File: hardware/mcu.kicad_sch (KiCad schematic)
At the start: 30 parts, among them J9 Conn_ARM_JTAG_SWD_10, Q1 MMBT3904, Q2 MMBT3904, Q3 MMBT3904, SW1 SW_Push, SW2 SW_Push, U3 STM32L476RGTx, Y1 DNP

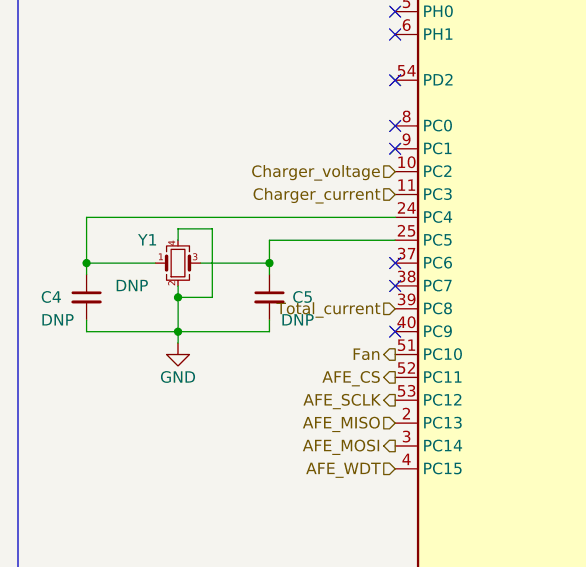
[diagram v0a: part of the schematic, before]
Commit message: Initiated sourcing
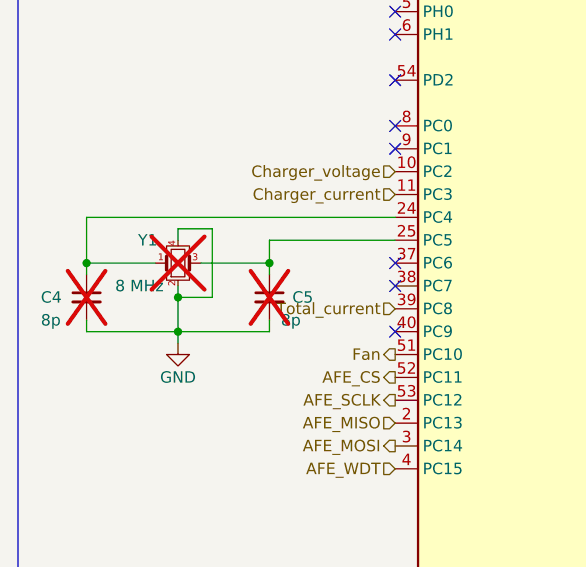
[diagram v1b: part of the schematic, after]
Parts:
- C4, C5: value DNP -> 8p; now not fitted
- Y1: value DNP -> 8 MHz; now not fitted
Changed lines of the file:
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@@
 		(in_bom yes)
 		(on_board yes)
-		(dnp no)
+		(dnp yes)
 		(property "Reference" "Y1"
 			(at 41.275 87.63 0)
@@
 			)
 		)
-		(property "Value" "DNP"
+		(property "Value" "8 MHz"
 			(at 38.735 92.71 0)
 			(effects
@@
 		(in_bom yes)
 		(on_board yes)
-		(dnp no)
+		(dnp yes)
 		(property "Reference" "C4"
 			(at 30.48 93.98 0)
@@
 			)
 		)
-		(property "Value" "DNP"
+		(property "Value" "8p"
 			(at 30.48 96.52 0)
 			(effects
@@
 		(in_bom yes)
 		(on_board yes)
-		(dnp no)
+		(dnp yes)
 		(property "Reference" "C5"
 			(at 58.42 93.98 0)
@@
 			)
 		)
-		(property "Value" "DNP"
+		(property "Value" "8p"
 			(at 57.15 96.52 0)
 			(effects

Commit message: More sourcing components
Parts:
- D1: footprint LED_THT:LED_D3.0mm -> LED_THT:LED_D5.0mm; LCSC (none) -> C2895548
- D2: footprint LED_THT:LED_D3.0mm -> LED_THT:LED_D5.0mm; LCSC (none) -> C2895492
- R2, R4, R7: footprint (none) -> Resistor_SMD:R_0402_1005Metric
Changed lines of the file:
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@@
 			)
 		)
-		(property "Footprint" ""
+		(property "Footprint" "Resistor_SMD:R_0402_1005Metric"
 			(at 247.65 144.78 0)
 			(effects
@@
 			)
 		)
-		(property "Footprint" "LED_THT:LED_D3.0mm"
+		(property "Footprint" "LED_THT:LED_D5.0mm"
 			(at 209.55 132.08 90)
 			(effects
@@
 		(property "Description" ""
 			(at 209.55 132.08 0)
+			(effects
+				(font
+					(size 1.27 1.27)
+				)
+				(hide yes)
+			)
+		)
+		(property "LCSC" "C2895492"
+			(at 209.55 132.08 90)
 			(effects
 				(font
@@
 			)
 		)
-		(property "Footprint" "LED_THT:LED_D3.0mm"
+		(property "Footprint" "LED_THT:LED_D5.0mm"
 			(at 171.45 132.08 90)
 			(effects
@@
 			)
 		)
+		(property "LCSC" "C2895548"
+			(at 171.45 132.08 90)
+			(effects
+				(font
+					(size 1.27 1.27)
+				)
+				(hide yes)
+			)
+		)
 		(pin "1"
 		)
@@
 			)
 		)
-		(property "Footprint" ""
+		(property "Footprint" "Resistor_SMD:R_0402_1005Metric"
 			(at 198.12 147.32 0)
 			(effects
@@
 			)
 		)
-		(property "Footprint" ""
+		(property "Footprint" "Resistor_SMD:R_0402_1005Metric"
 			(at 160.02 147.32 0)
 			(effects

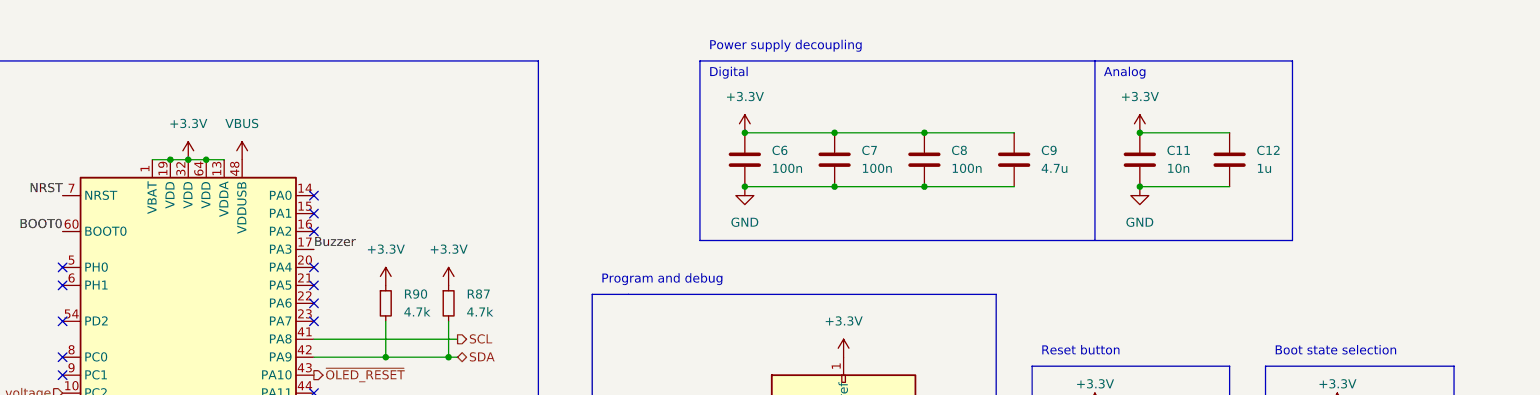
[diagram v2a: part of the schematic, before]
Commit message: Improved Currrent Sensors
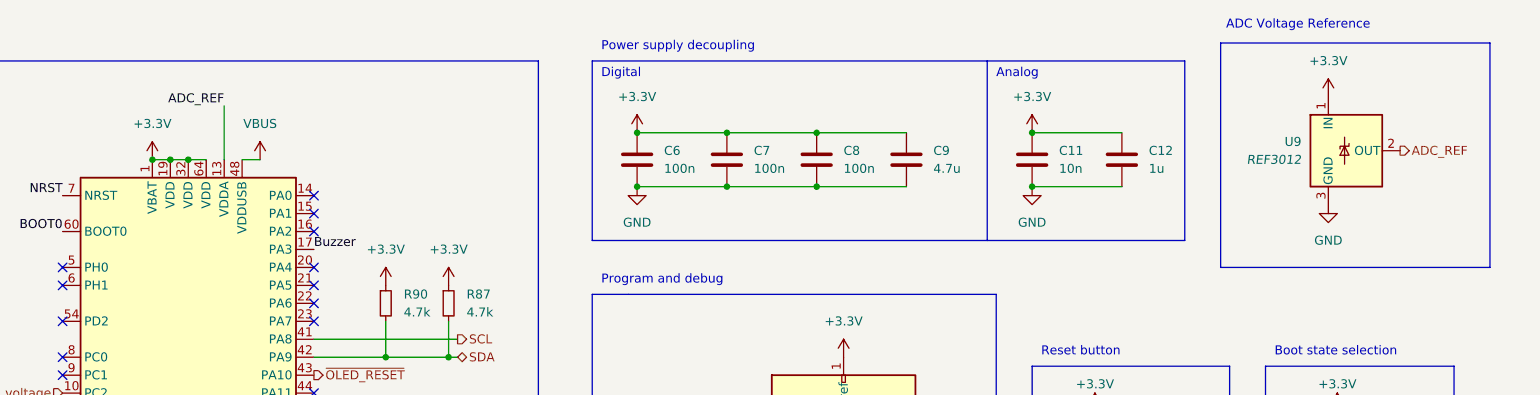
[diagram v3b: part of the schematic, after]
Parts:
- added U9: REF3012, Package_TO_SOT_SMD:SOT-23, symbol Reference_Voltage:REF3012
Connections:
- net +3.3V: now also U9.1 (IN); no longer U3.13 (VDDA)
- net GND: now also U9.3 (GND)
- new net ADC_REF: U3.13 (VDDA), U9.2 (OUT)
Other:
- note added: "ADC Voltage Reference"
- moved on the sheet: C11, C12, C6, C7, C8, C9

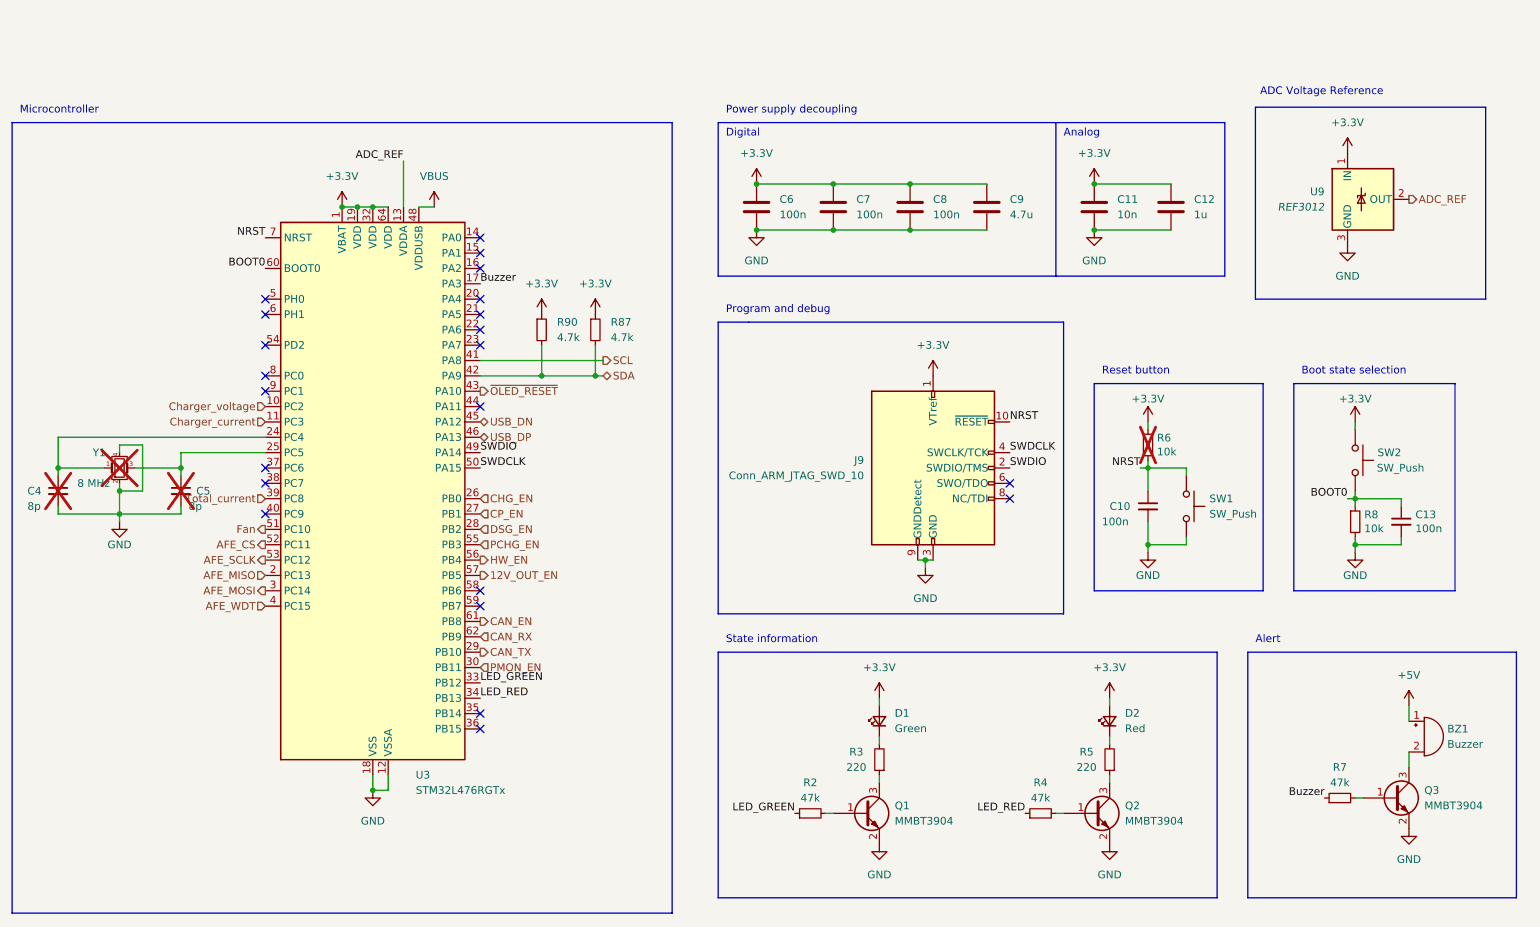
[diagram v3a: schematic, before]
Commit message: Charger monitoring
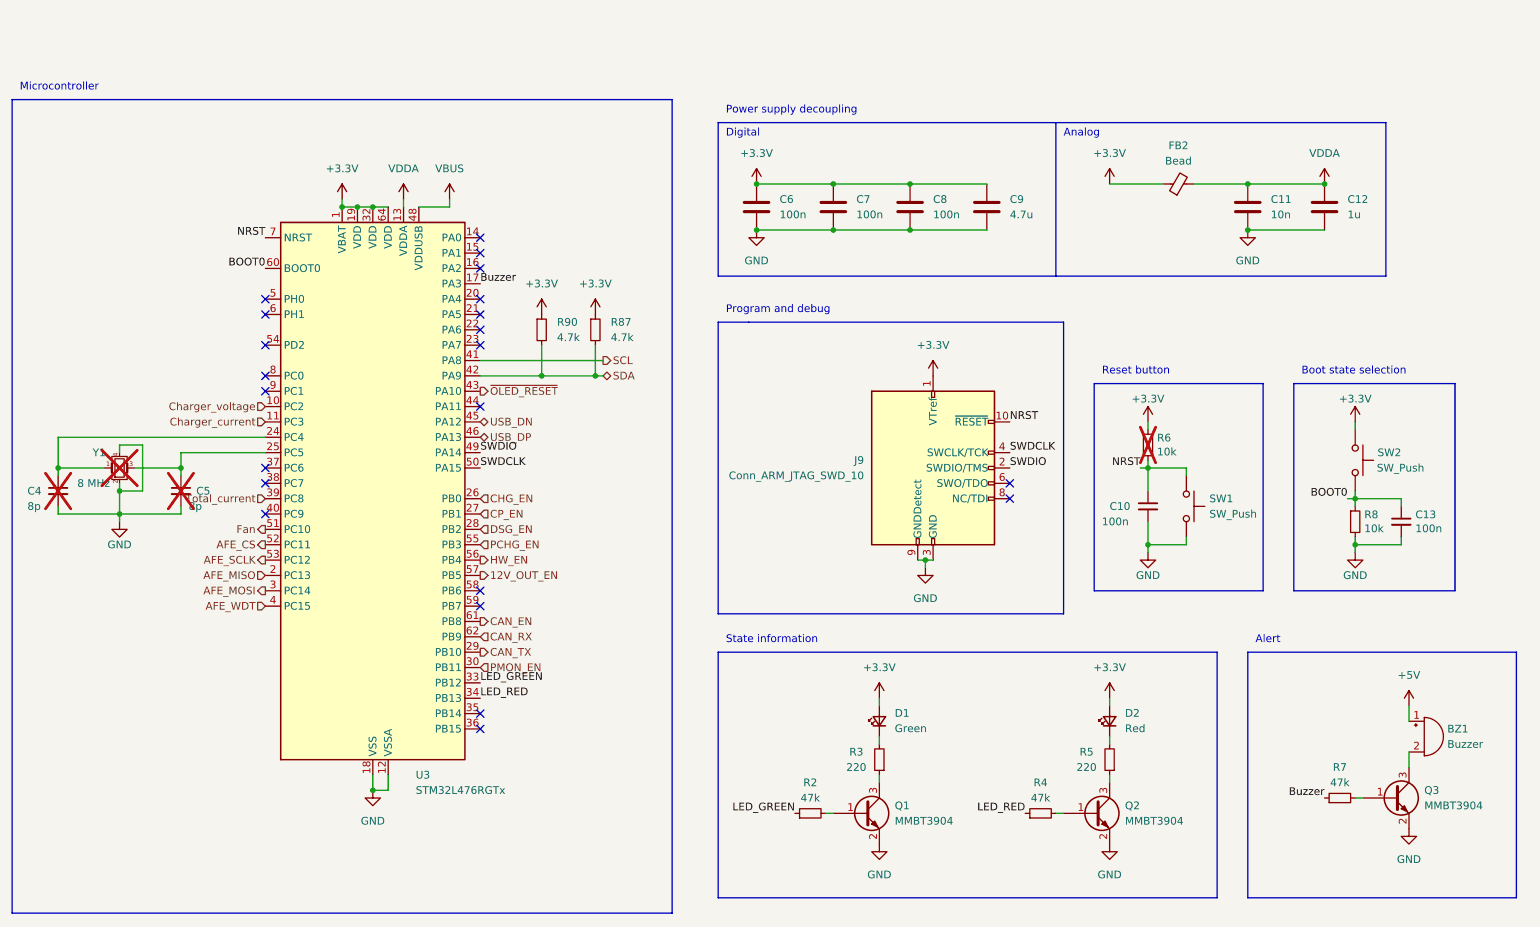
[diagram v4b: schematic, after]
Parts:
- removed U9: REF3012, Package_TO_SOT_SMD:SOT-23, symbol Reference_Voltage:REF3012
- added FB2: Bead, symbol Device:FerriteBead_Small
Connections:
- net +3.3V: now also FB2.1; no longer C11.1, C12.1
- net ADC_REF renamed VDDA
- net VDDA: now also C11.1, C12.1, FB2.2
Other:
- note removed: "ADC Voltage Reference"
- moved on the sheet: C11, C12

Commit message: Changed MCU and AFE
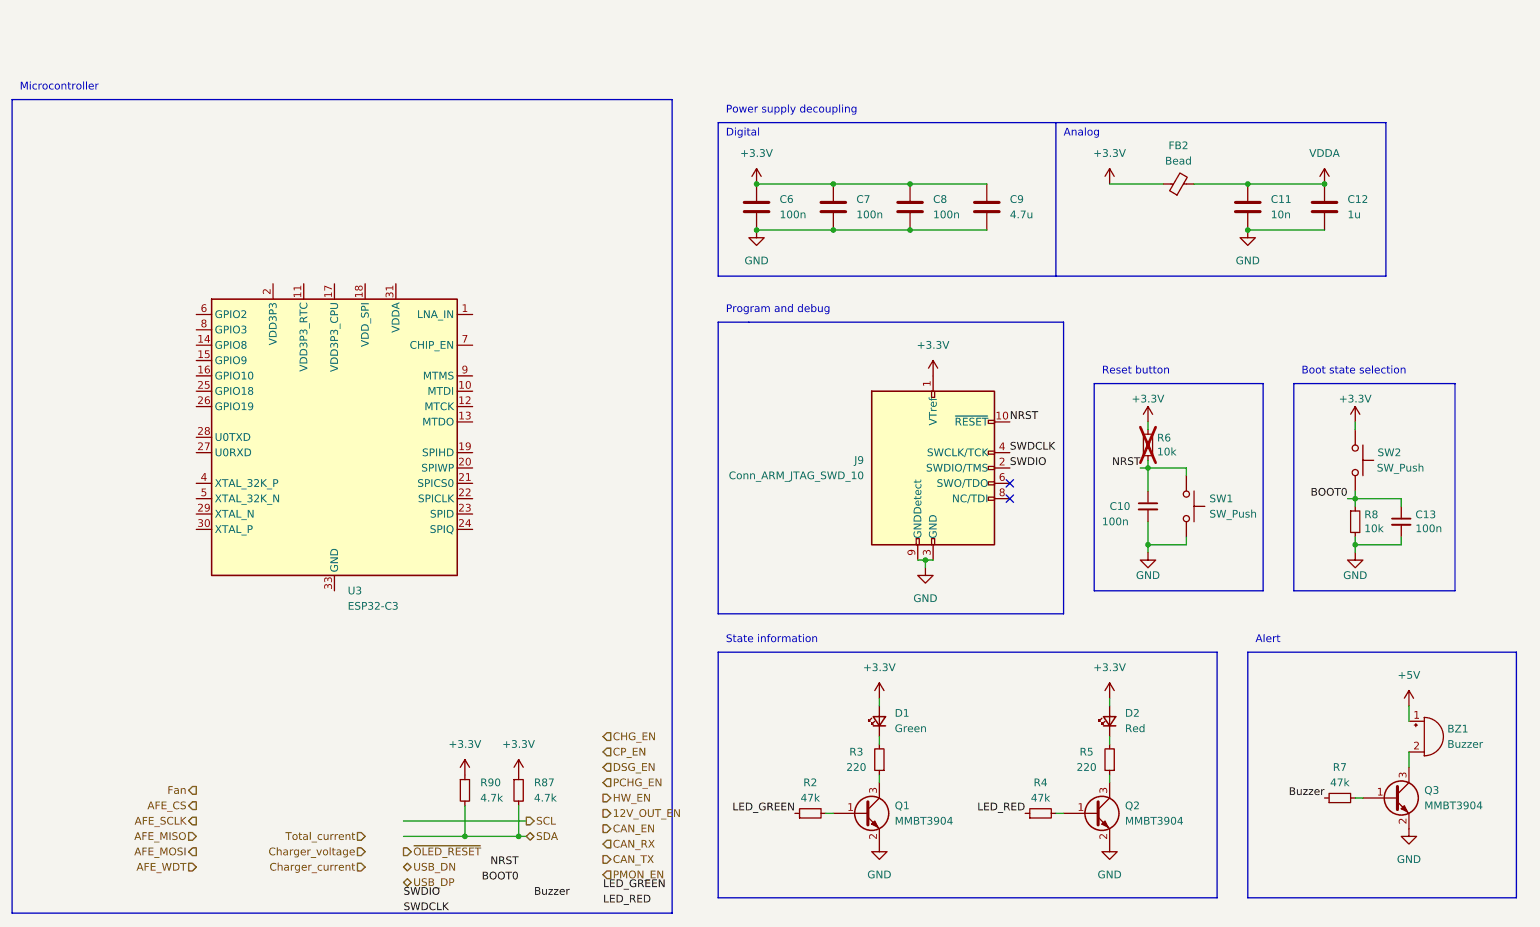
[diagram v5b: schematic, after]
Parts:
- removed C4, C5: 8p, Capacitor_SMD:C_0402_1005Metric, symbol Device:C_Small
- removed U3: STM32L476RGTx, Package_QFP:LQFP-64_10x10mm_P0.5mm, symbol MCU_ST_STM32L4:STM32L476RGTx
- removed Y1: 8 MHz, Crystal:Crystal_SMD_3225-4Pin_3.2x2.5mm, symbol Device:Crystal_GND24_Small
- added U3: ESP32-C3, Package_DFN_QFN:QFN-32-1EP_5x5mm_P0.5mm_EP3.7x3.7mm, symbol MCU_Espressif:ESP32-C3
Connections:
- new net: U3.2 (VDD3P3), U3.3 (VDD3P3)
- new net: U3.31 (VDDA), U3.32 (VDDA)
- no-connect marks 22 -> 2
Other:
- moved on the sheet: R87, R90

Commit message: Remove uneeded peripherals
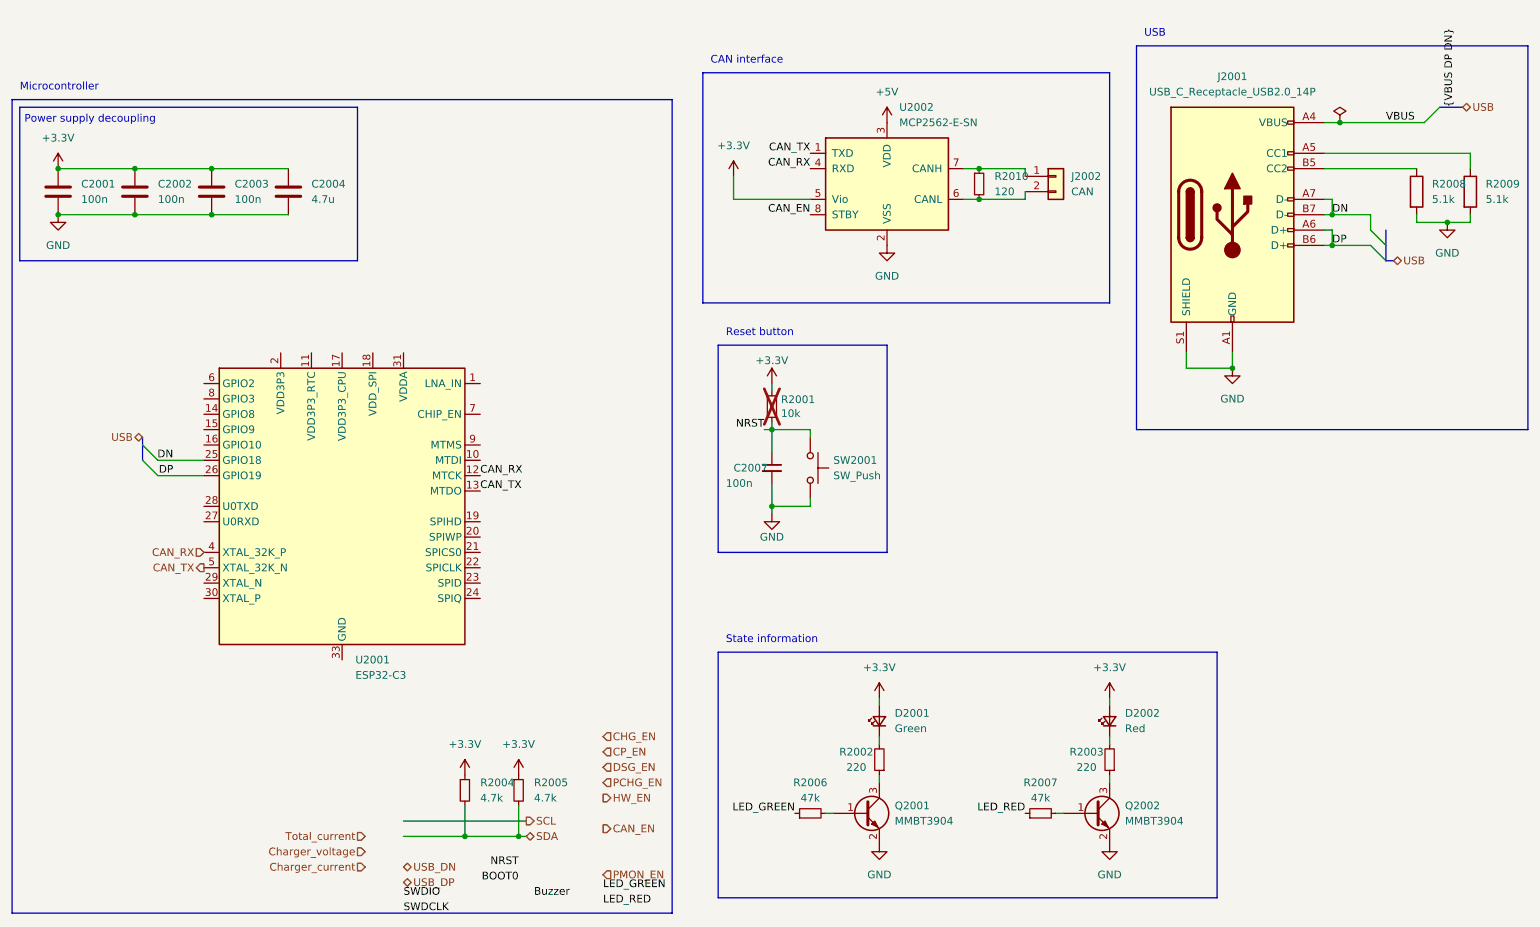
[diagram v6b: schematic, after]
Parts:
- removed BZ1: Buzzer, symbol Device:Buzzer
- removed C11: 10n, Capacitor_SMD:C_0402_1005Metric, symbol Device:C
- removed C12: 1u, Capacitor_SMD:C_0402_1005Metric, symbol Device:C
- removed C13: 100n, Capacitor_SMD:C_0402_1005Metric, symbol Device:C_Small
- removed FB2: Bead, symbol Device:FerriteBead_Small
- removed J9: Conn_ARM_JTAG_SWD_10, Connector_PinHeader_1.27mm:PinHeader_2x05_P1.27mm_Vertical_SMD, symbol Connector:Conn_ARM_JTAG_SWD_10
- removed Q3: MMBT3904, Package_TO_SOT_SMD:SOT-23, symbol Transistor_BJT:MMBT3904
- removed R7: 47k, Resistor_SMD:R_0402_1005Metric, symbol Device:R_Small
- removed R8: 10k, Resistor_SMD:R_0603_1608Metric, symbol Device:R_Small
- removed SW2: SW_Push, Button_Switch_SMD:SW_SPST_CK_RS282G05A3, symbol Switch:SW_Push
- added J2001: USB_C_Receptacle_USB2.0_14P, Connector_USB:USB_C_Receptacle_Palconn_UTC16-G, symbol Connector:USB_C_Receptacle_USB2.0_14P
- added J2002: CAN, Connector_Phoenix_MC:PhoenixContact_MCV_1,5_2-G-3.5_1x02_P3.50mm_Vertical, symbol Connector_Generic:Conn_01x02
- added R2008, R2009: 5.1k, Resistor_SMD:R_0603_1608Metric, symbol Device:R
- added R2010: 120, Resistor_SMD:R_0603_1608Metric, symbol Device:R_Small
- added U2002: MCP2562-E-SN, Package_SO:SOIC-8_3.9x4.9mm_P1.27mm, symbol Interface_CAN_LIN:MCP2562-E-SN
- renumbered C6 to C2001, C7 to C2002, C8 to C2003, C9 to C2004, C10 to C2007, D1 to D2001, D2 to D2002, Q1 to Q2001, Q2 to Q2002, R6 to R2001, R3 to R2002, R5 to R2003, R90 to R2004, R87 to R2005, R2 to R2006, R4 to R2007, SW1 to SW2001, U3 to U2001
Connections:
- net +3.3V: now also U2002.5 (Vio)
- net +5V: now also U2002.3 (VDD)
- net CAN_EN: now also U2002.8 (STBY)
- net CAN_RX: now also U2001.12 (MTCK), U2001.4 (XTAL_32K_P), U2002.4 (RXD)
- net CAN_TX: now also U2001.13 (MTDO), U2001.5 (XTAL_32K_N), U2002.1 (TXD)
- net GND: now also J2001.A1 (GND), J2001.A12 (GND), J2001.B1 (GND), J2001.B12 (GND), J2001.S1 (SHIELD), R2008.2, R2009.2, U2002.2 (VSS)
- net DN: now reaches U2001.25 (GPIO18)
- net DN: now also J2001.A7 (D-), J2001.B7 (D-)
- net DP: now reaches U2001.26 (GPIO19)
- net DP: now also J2001.A6 (D+), J2001.B6 (D+)
- new net: J2001.A5 (CC1), R2009.1
- new net: J2001.B5 (CC2), R2008.1
- new net: J2002.2 (Pin_2), R2010.2, U2002.6 (CANL)
- new net: J2002.1 (Pin_1), R2010.1, U2002.7 (CANH)
- new net VBUS: J2001.A4 (VBUS), J2001.A9 (VBUS), J2001.B4 (VBUS), J2001.B9 (VBUS)
- no-connect marks 2 -> 0
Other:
- note added: "CAN interface"
- note added: "USB"
- note removed: "Alert"
- note removed: "Analog"
- note removed: "Boot state selection"
- note removed: "Digital"
- note removed: "Program and debug"
- moved on the sheet: C2001, C2002, C2003, C2004, C2007, R2001, SW2001, U2001
